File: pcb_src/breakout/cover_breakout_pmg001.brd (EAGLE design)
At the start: 25.4 x 60.3 mm, 0 parts

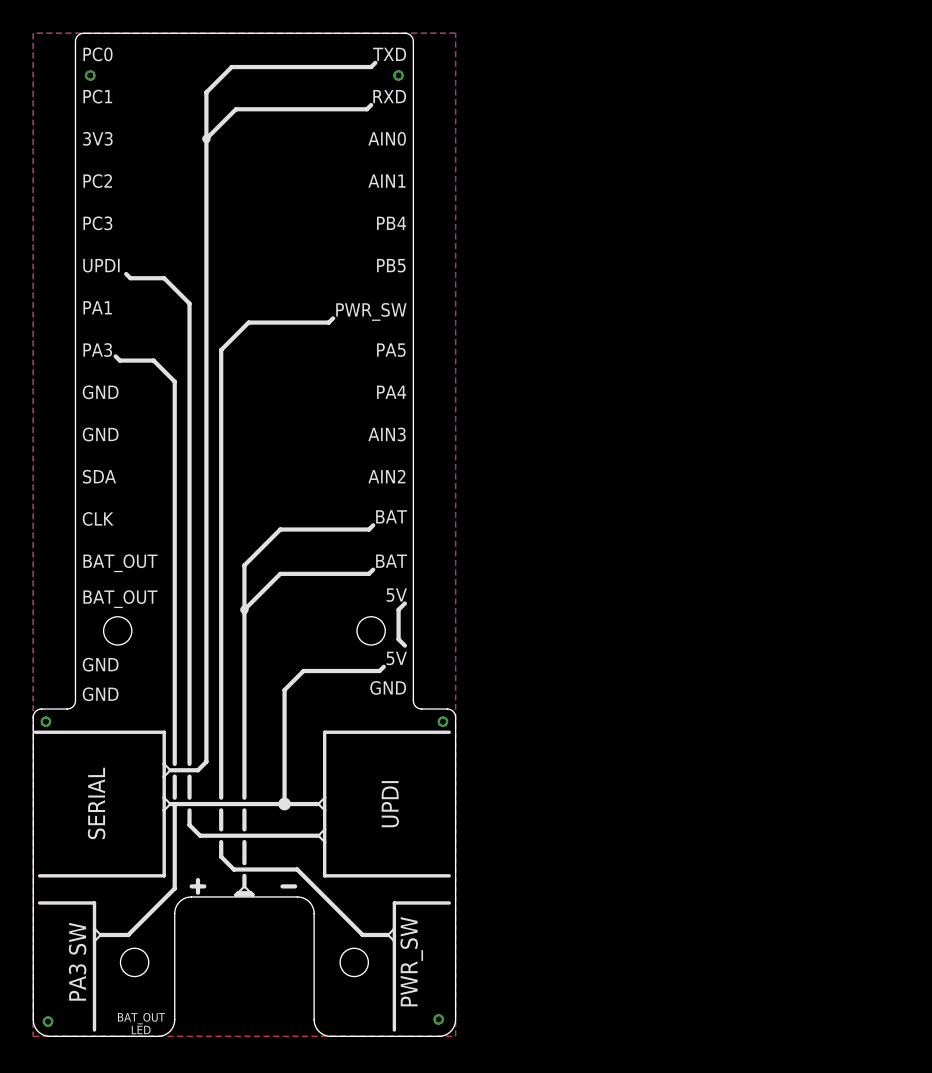
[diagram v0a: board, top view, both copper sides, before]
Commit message: Reworked repository
Name changed, added a lot of new resources etc.
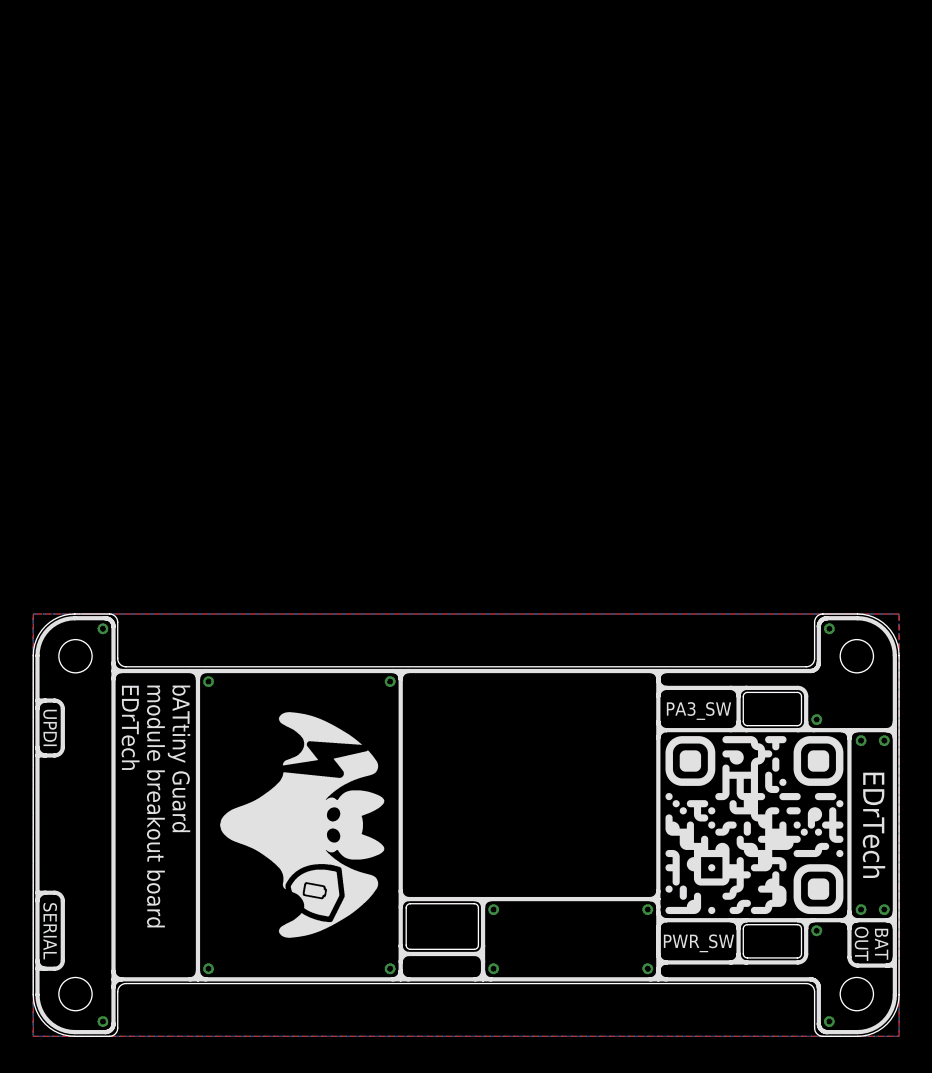
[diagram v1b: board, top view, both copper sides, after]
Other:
- board size 25.4 x 60.3 mm -> 52.1 x 25.4 mm
- board text added: "BAT OUT"
- board text added: "EDrTech"
- board text added: "PA3_SW"
- board text added: "bATtiny Guard module breakout board EDrTech"
- board text removed: "3V3"
- board text removed: "5V"
- board text removed: "AIN0"
- board text removed: "AIN1"
- board text removed: "AIN2"
- board text removed: "AIN3"
- board text removed: "BAT"
- board text removed: "BAT_OUT"
- board text removed: "BAT_OUT LED"
- board text removed: "CLK"
- board text removed: "EDrTech PMG001 Breakout"
- board text removed: "GND"
- board text removed: "PA1"
- board text removed: "PA3"
- board text removed: "PA3 SW"
- board text removed: "PA4"
- board text removed: "PA5"
- board text removed: "PB4"
- board text removed: "PB5"
- board text removed: "PC0"
- board text removed: "PC1"
- board text removed: "PC2"
- board text removed: "PC3"
- board text removed: "RXD"
- board text removed: "SDA"
- board text removed: "TXD"
